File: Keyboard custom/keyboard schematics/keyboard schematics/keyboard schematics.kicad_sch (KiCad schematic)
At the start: 1 part, among them U1 ATmega32U4-A

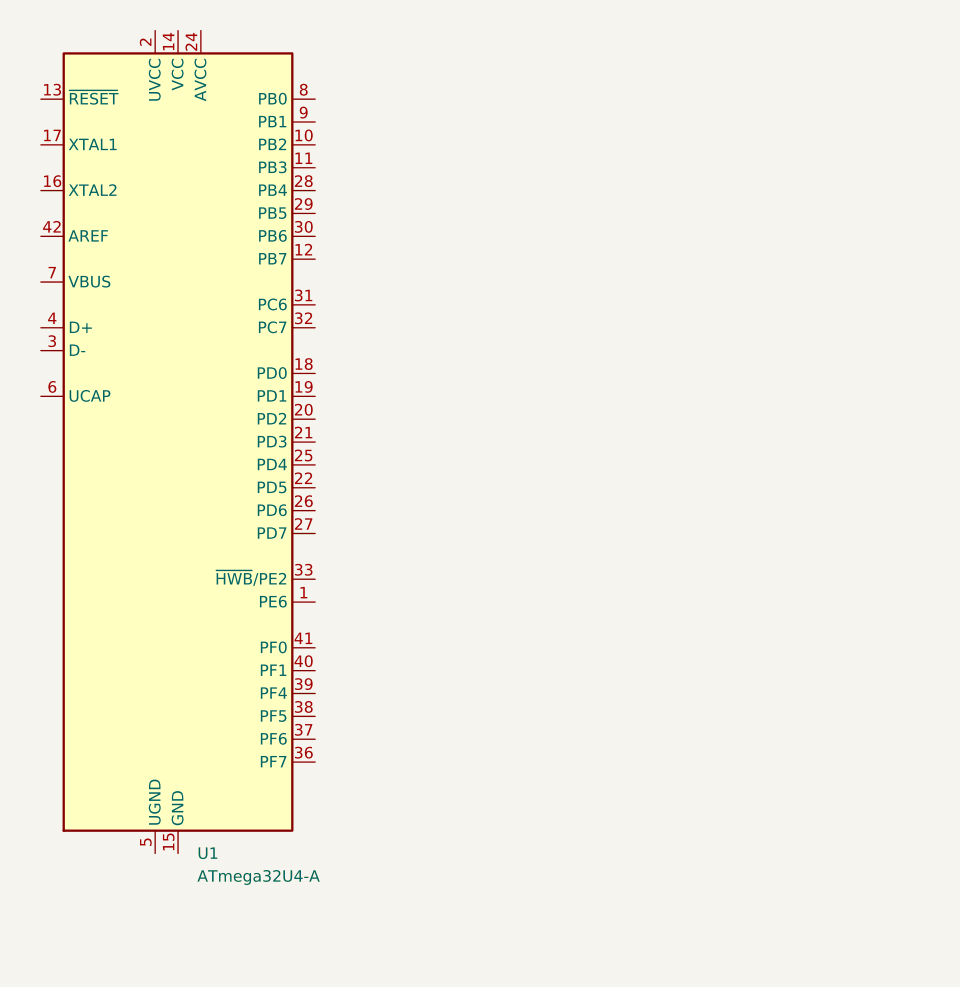
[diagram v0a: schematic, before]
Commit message: schematics progres
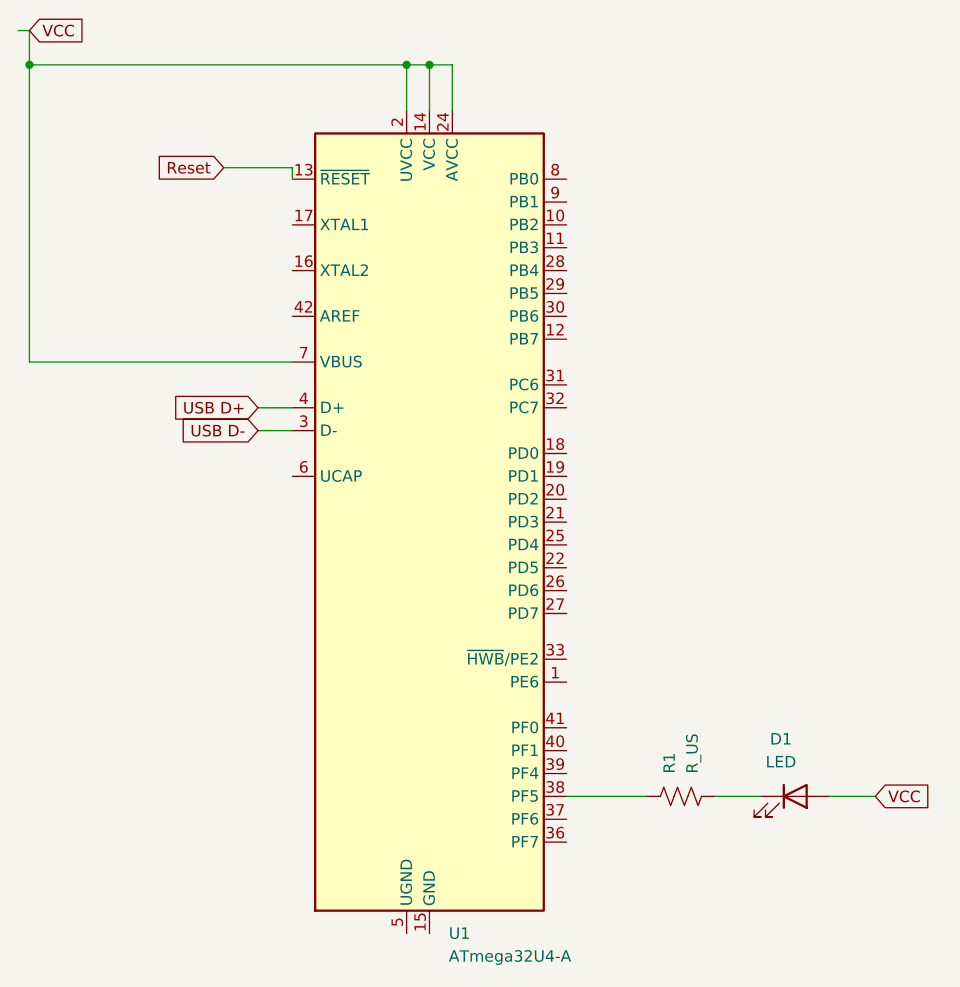
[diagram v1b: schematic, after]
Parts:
- added D1: LED, symbol Device:LED
- added R1: R_US, symbol Device:R_US
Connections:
- net Reset: now reaches U1.13 (~{RESET})
- net VCC: now reaches U1.14 (VCC), U1.34 (VCC)
- net VCC: now also U1.2 (UVCC), U1.24 (AVCC), U1.44 (AVCC), U1.7 (VBUS), D1.2 (A)
- net USB D-: now reaches U1.3 (D-)
- net at U1.38 (PF5): now also R1.1
- net USB D+: now reaches U1.4 (D+)
- new net: D1.1 (K), R1.2
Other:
- moved on the sheet: U1
